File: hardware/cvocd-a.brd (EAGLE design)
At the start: 152.5 x 43.6 mm, 78 parts, among them IC1 6N138, IC2 LM324D, IC3 MCP4728_QUAD_DAC, IC4 REG1117, IC5 PIC16F1825SO14, IC6 74HC595D, IC7 74HC595D

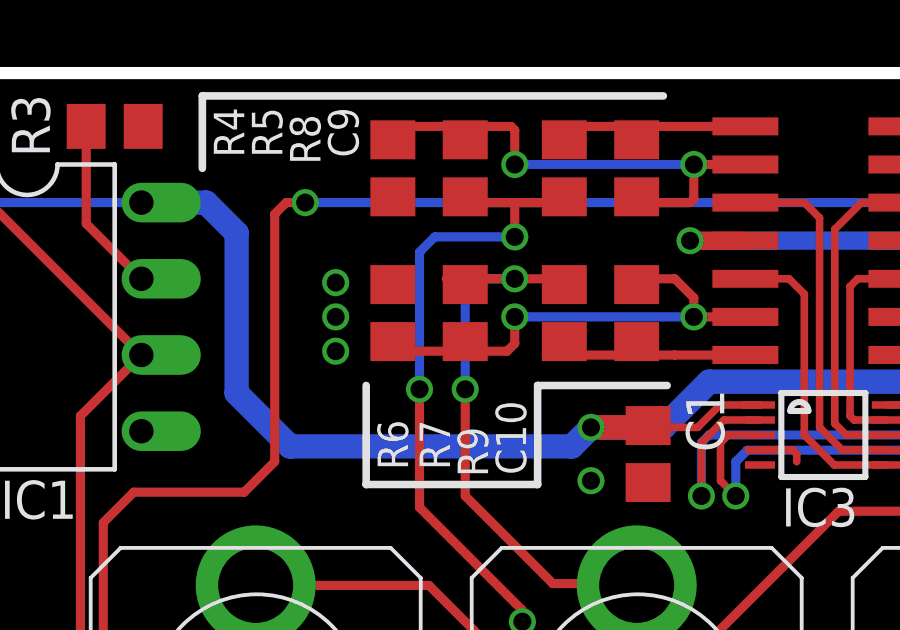
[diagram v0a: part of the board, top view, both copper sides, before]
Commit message: v5 pcb release candidate
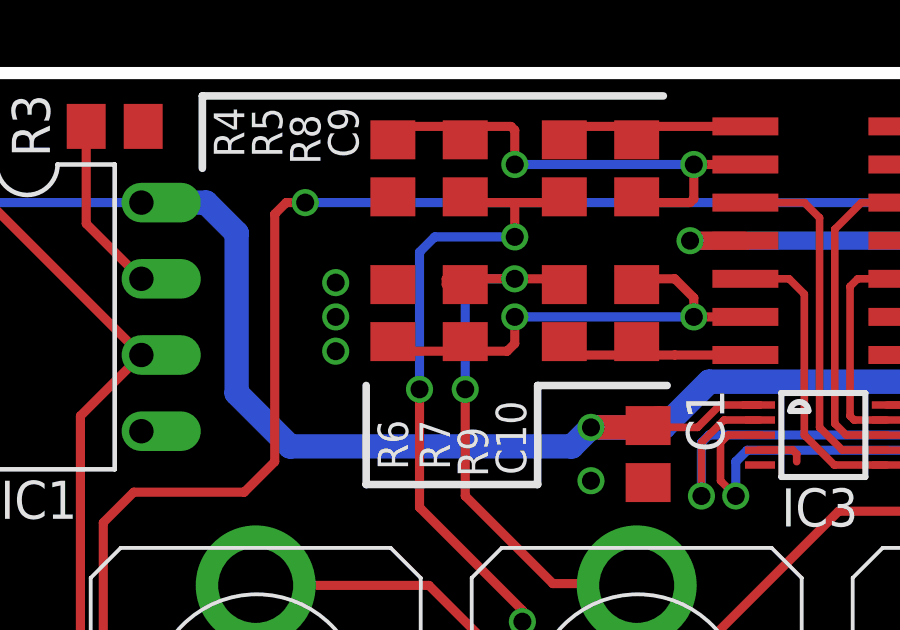
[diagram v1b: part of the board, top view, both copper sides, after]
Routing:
- net N$19: track 19.9 -> 20.7 mm
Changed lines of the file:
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@@
 <wire x1="49.723" y1="35.56" x2="49.53" y2="35.367" width="0.3048" layer="1"/>
 <wire x1="41.402" y1="33.467" x2="41.402" y2="33.147" width="0.3048" layer="1"/>
-<wire x1="41.402" y1="33.147" x2="45.212" y2="33.147" width="0.3048" layer="1"/>
+<wire x1="41.402" y1="33.147" x2="43.815" y2="33.147" width="0.3048" layer="1"/>
 <wire x1="45.212" y1="33.147" x2="45.466" y2="33.401" width="0.3048" layer="1"/>
 <wire x1="45.466" y1="33.401" x2="45.466" y2="34.29" width="0.3048" layer="1"/>
-<wire x1="45.212" y1="33.147" x2="43.815" y2="33.467" width="0" layer="19" extent="1-1"/>
+<wire x1="45.212" y1="33.147" x2="43.815" y2="33.147" width="0.3048" layer="1"/>
+<wire x1="43.815" y1="33.147" x2="43.815" y2="33.467" width="0.3048" layer="1"/>
 </signal>
 <signal name="VOUTA">
@@
 <wire x1="46.736" y1="25.4" x2="49.47" y2="25.4" width="0.3048" layer="1"/>
 <wire x1="49.47" y1="25.4" x2="49.53" y2="25.34" width="0.3048" layer="1"/>
-<wire x1="43.815" y1="35.052" x2="43.815" y2="35.367" width="0" layer="19" extent="1-16"/>
+<wire x1="43.815" y1="35.367" x2="43.18" y2="35.367" width="0.3048" layer="1"/>
+<wire x1="43.18" y1="35.367" x2="43.18" y2="35.56" width="0.3048" layer="1"/>
 </signal>
 <signal name="N$38">
